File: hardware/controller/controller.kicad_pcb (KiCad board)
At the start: 4 copper layers, 77 parts, among them J1 USB_C_Receptacle_USB2.0_16P, J2 Micro_SD_Card_Det_Hirose_DM3AT, J3 Display, SW1 Reset, SW2 Boot, SW3 SW_SPDT, SW4 EStop, U2 SX1262IMLTRT, U3 MP2672AGD-0000-Z, U4 PE4259, U5 LMR51625XDDCR, U6 ESP32-S3-MINI-1, Y2 32MHz

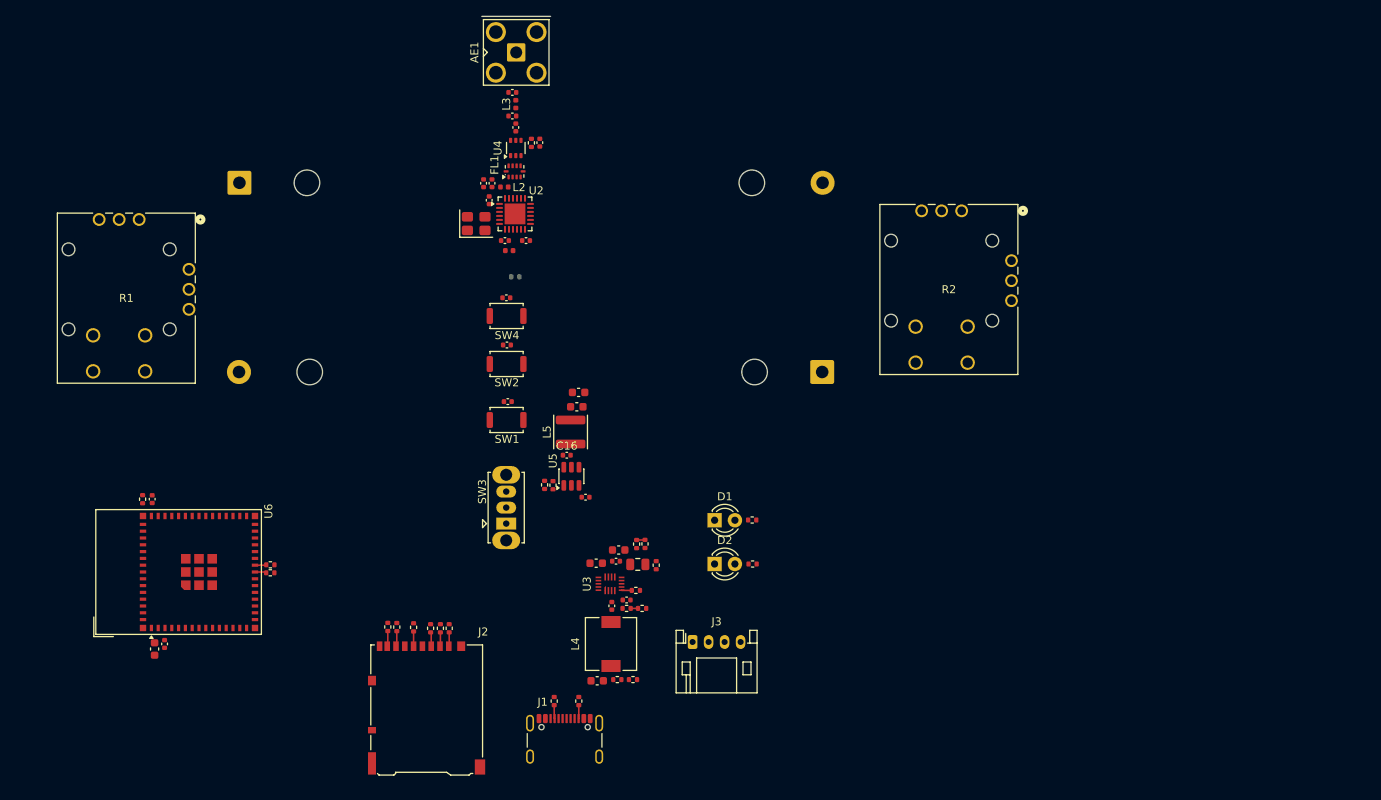
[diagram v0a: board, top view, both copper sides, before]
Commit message: routing board
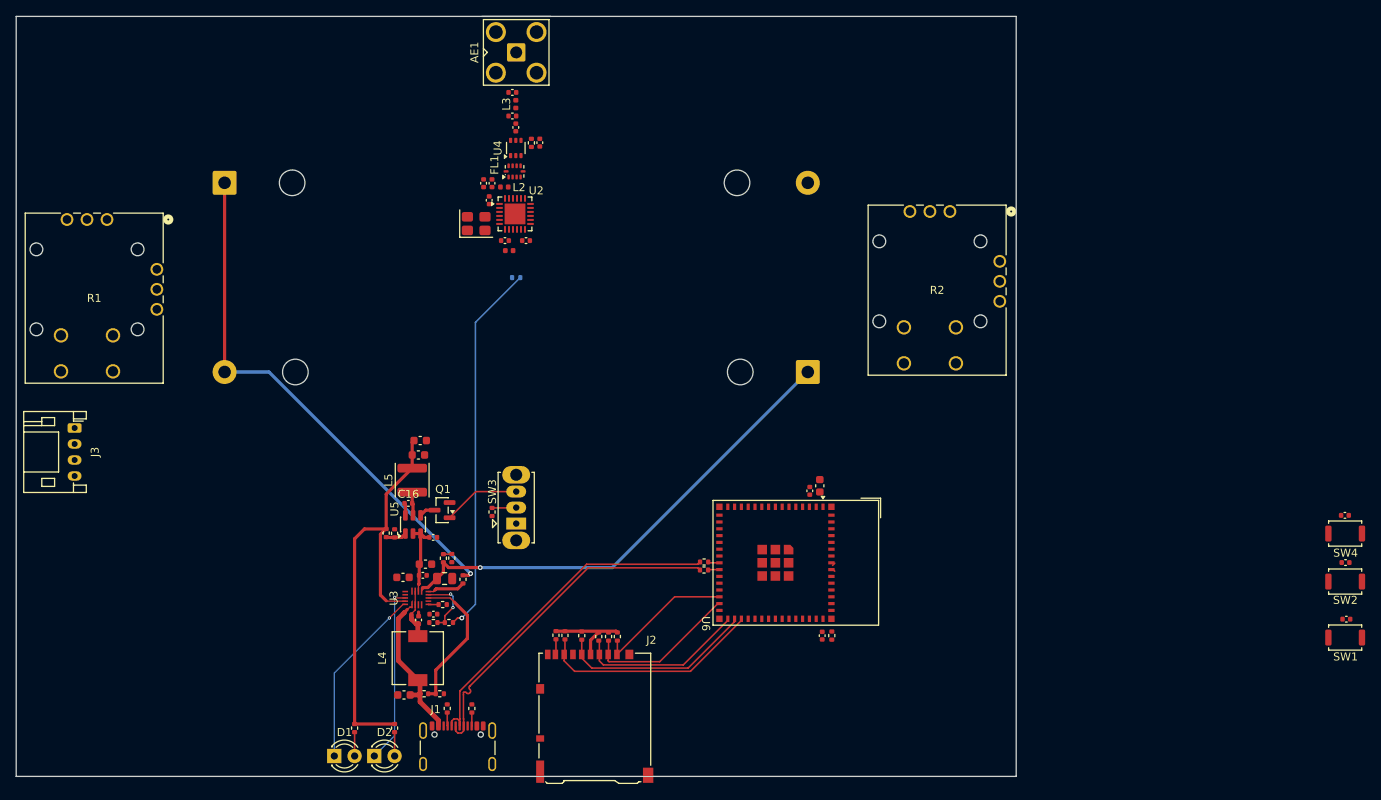
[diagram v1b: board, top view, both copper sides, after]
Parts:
- added Q1: AO3400A, Package_TO_SOT_SMD:SOT-23, F.Cu at (133.9, 126.3)
- added R27: 10K, Resistor_SMD:R_0402_1005Metric, F.Cu at (140.2, 126.5)
- moved C13 108.3 mm to (246.9, 132.8)
- moved C26 108.3 mm to (246.8, 126.9)
- moved SW1 108.3 mm to (246.8, 142.2)
- moved SW2 108.3 mm to (246.8, 135.2)
- moved SW4 108.3 mm to (246.8, 129.2)
- moved C14 108.3 mm to (247.0, 139.9)
- moved R3 87.8 mm to (182.7, 141.9), turned to 90 degrees
- moved C6 85.6 mm to (181.2, 123.2), turned to 90 degrees
- moved C4 85.5 mm to (181.4, 142.0), turned to 90 degrees
- moved C5 82.9 mm to (179.9, 123.9), turned to 90 degrees
- moved J3 81.8 mm to (88.0, 116.0), turned to -90 degrees
- moved U6 77.2 mm to (178.2, 132.8), turned to -90 degrees
- moved R15 56.1 mm to (123.0, 153.5), turned to -90 degrees
- moved D1 55.9 mm to (120.5, 157.0)
- moved R25 54.2 mm to (166.7, 132.8), turned to 180 degrees
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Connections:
- C15 pad 1: Net-(SW3-C) -> VCC
- R1 pad A: unconnected-(R1-PadA) -> /JOY_1_BTN
- R1 pad B: GND -> unconnected-(R1-PadB)
- R1 pad C: /JOY_1_BTN -> unconnected-(R1-PadC)
- R1 pad D: unconnected-(R1-PadD) -> GND
- R2 pad A: unconnected-(R2-PadA) -> /JOY_2_BTN
- R2 pad B: GND -> unconnected-(R2-PadB)
- R2 pad C: /JOY_2_BTN -> unconnected-(R2-PadC)
- R2 pad D: unconnected-(R2-PadD) -> GND
- SW3 pad 2: VCC -> Net-(SW3-B)
- SW3 pad 3: Net-(SW3-C) -> Net-(Q1-G)
- U5 pad 2: Net-(SW3-C) -> VCC
- U5 pad 3: Net-(SW3-C) -> VCC
- U5 pad 4: GND -> Net-(Q1-D)
- U6 pad 14: unconnected-(U6-IO10-Pad14) -> /SX_CS
- U6 pad 15: unconnected-(U6-IO11-Pad15) -> /MOSI
- U6 pad 16: unconnected-(U6-IO12-Pad16) -> /SCK
- U6 pad 17: unconnected-(U6-IO13-Pad17) -> /MISO
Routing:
- net +3.3V: track 0.00 -> 68.1 mm
- net Net-(BT1--): track 0.00 -> 65.9 mm, vias 0 -> 1
- net Net-(BT1-+): track 0.00 -> 61.0 mm, vias 0 -> 1
- net Net-(R19-Pad2): track 0.00 -> 46.9 mm, vias 0 -> 1
- net /USB_D-: track 0.00 -> 43.5 mm
- net /USB_D+: track 0.00 -> 43.5 mm
- net /SD_DAT0: track 1.92 -> 28.3 mm
- net /SD_CLK: track 1.84 -> 24.7 mm
- net Net-(D1-K): track 0.00 -> 22.8 mm, vias 0 -> 1
- net Net-(D2-K): track 0.00 -> 22.2 mm, vias 0 -> 1
- net /SD_CMD: track 1.76 -> 21.3 mm
- net VBUS: track 0.00 -> 19.3 mm
- net Net-(U3-VLIM): track 0.00 -> 18.2 mm
- net /SD_DAT3: track 1.75 -> 19.5 mm
- net /SD_DAT2: track 1.75 -> 17.5 mm
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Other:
- board outline added: 125 x 95 mm
